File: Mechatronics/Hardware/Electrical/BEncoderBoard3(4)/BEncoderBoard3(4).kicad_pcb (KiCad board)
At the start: 2 copper layers, 8.5 x 13 mm, 5 parts, among them J1 Conn_01x06_Male, U9 LSM6DSRX

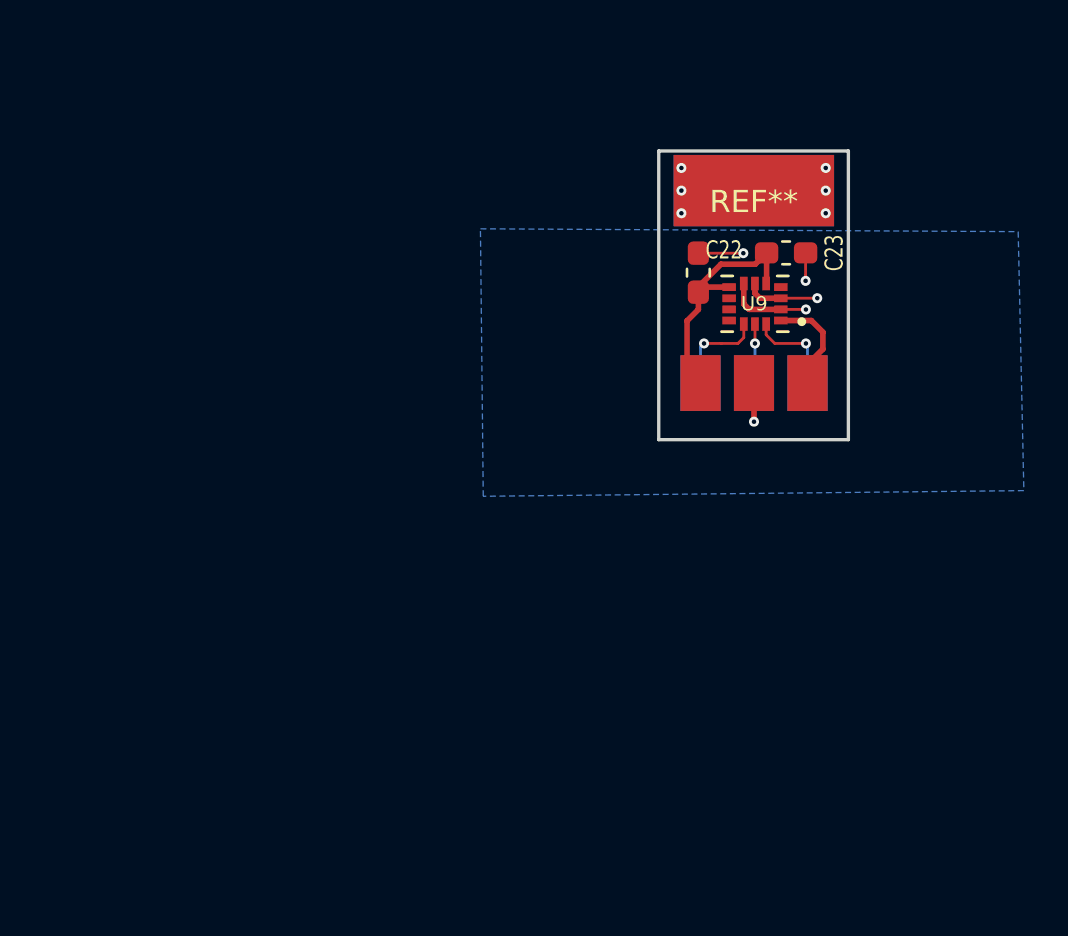
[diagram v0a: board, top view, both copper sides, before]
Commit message: PCB changes
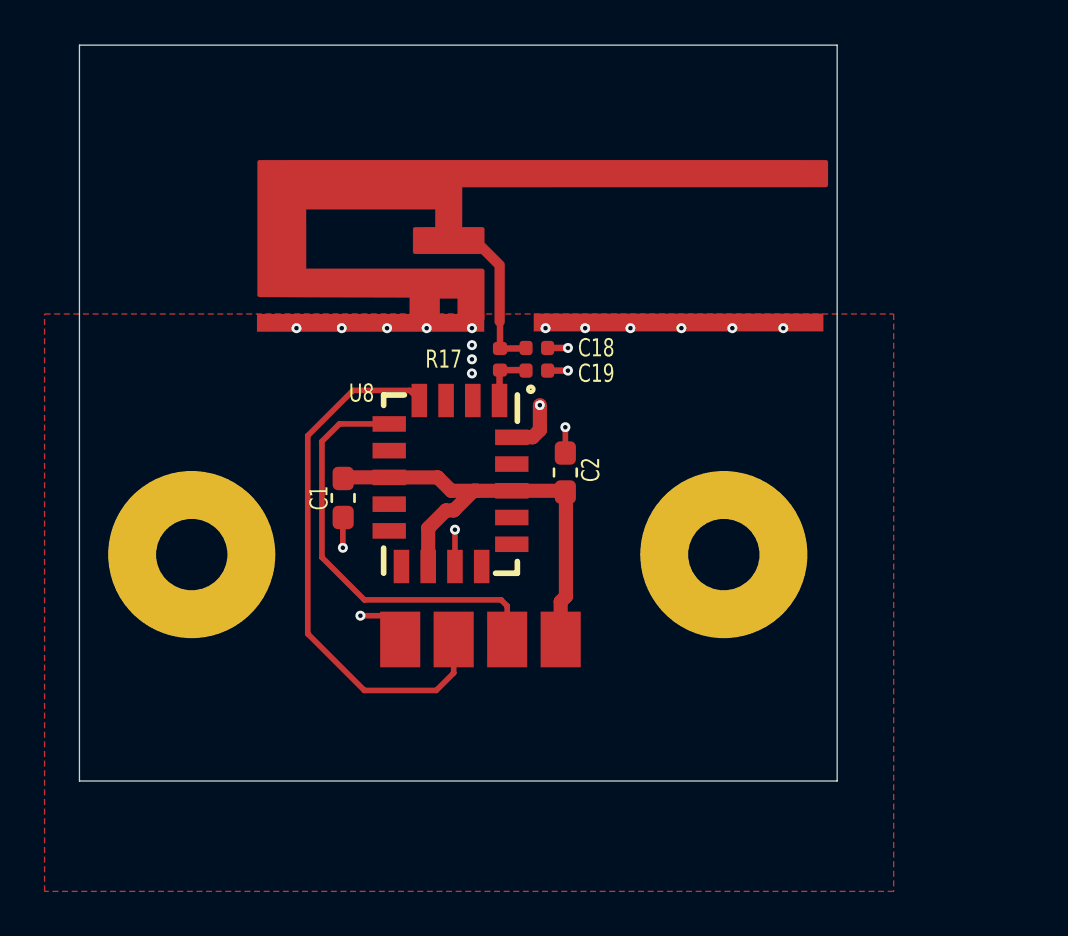
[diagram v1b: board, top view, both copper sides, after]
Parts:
- removed C22, C23: 100nF, Encoder:C_0603_1608Metric_Pad1.05x0.95mm_HandSolder
- removed the REF** at (146.8, 83.5)
- removed U9: LSM6DSRX, Encoder:LSM6DSRX
- added AE1: LOGO, Encoder:Antenna, F.Cu at (137.3, 85.9)
- added C1: 1uF, Encoder:C_0603_1608Metric_Pad1.05x0.95mm_HandSolder, F.Cu at (128.3, 97.3)
- added C18: C_Rf, Encoder:C_0402_1005Metric, F.Cu at (137.0, 90.6)
- added C19: C_Rf, Encoder:C_0402_1005Metric, F.Cu at (137.0, 91.6)
- added C2: 10uF, Encoder:C_0603_1608Metric_Pad1.05x0.95mm_HandSolder, F.Cu at (138.3, 96.1)
- added R17: L_Rf, Encoder:L_0402_1005Metric, F.Cu at (135.4, 91.1)
- added REF**: MountingHole_3.2mm_M3_Pad, Encoder:MountingHole_3.2mm_M3_Pad, F.Cu at (121.5, 99.8)
- added U8: RN4871U, Encoder:RN4871U, F.Cu at (130.1, 92.7)
- added e: MountingHole_3.2mm_M3_Pad, Encoder:MountingHole_3.2mm_M3_Pad, F.Cu at (145.4, 99.8)
- J1: value Conn_01x06_Male -> Conn_01x04_Male; footprint Encoder:SolderWirePad_1x06_SMD_5x10mm -> Encoder:SolderWirePad_1x04_SMD_5x10mm_copy
- moved J1 16.9 mm to (134.5, 103.6)
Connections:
- J1 pad 1: /CS -> GND
- J1 pad 2: /SCL -> Net-(J1-Pad2)
- J1 pad 3: /SDA -> Net-(J1-Pad3)
- J1 pad 4: /SDO -> +3V3
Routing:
- net Net-(J1-Pad2): track 0.00 -> 24.4 mm
- net Net-(J1-Pad3): track 0.00 -> 19.3 mm
- net +3V3: track 11.3 -> 21.7 mm
- net /SDO: track 4.68 -> 0.00 mm
- net /CS: track 4.34 -> 0.00 mm, vias 1 -> 0
- net /SDA: track 4.23 -> 0.00 mm, vias 1 -> 0
- net /SCL: track 2.66 -> 0.00 mm, vias 1 -> 0
- net Net-(C19-Pad1): track 0.00 -> 2.60 mm
- net Net-(AE1-Pad1): track 0.00 -> 2.33 mm
- net GND: track 12.1 -> 11.0 mm, vias 5 -> 21
- net (no net): vias 6 -> 0
- added copper zone on F.Cu, net GND
- added copper zone on In1.Cu, net GND
- removed copper zone on B.Cu, net GND
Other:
- board size 8.5 x 13 mm -> 34 x 33 mm
- copper layers 2 -> 4
- net class Default: clearance 0.127 -> 0.1016; trace_width 0.127 -> 0.1016
- rule trace_clearance: 0.127 -> 0.1016
- rule trace_min: 0.127 -> 0.0889
- rule via_min_size: 0.45 -> 0.44
